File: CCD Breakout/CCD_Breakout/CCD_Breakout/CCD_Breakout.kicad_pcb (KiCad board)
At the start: 2 copper layers, 80.5 x 25.4 mm, 33 parts, among them U1 CCD, U3 ADC-MCP33151, U5 74HC541PW_118, U8 OPA4322AIPWR

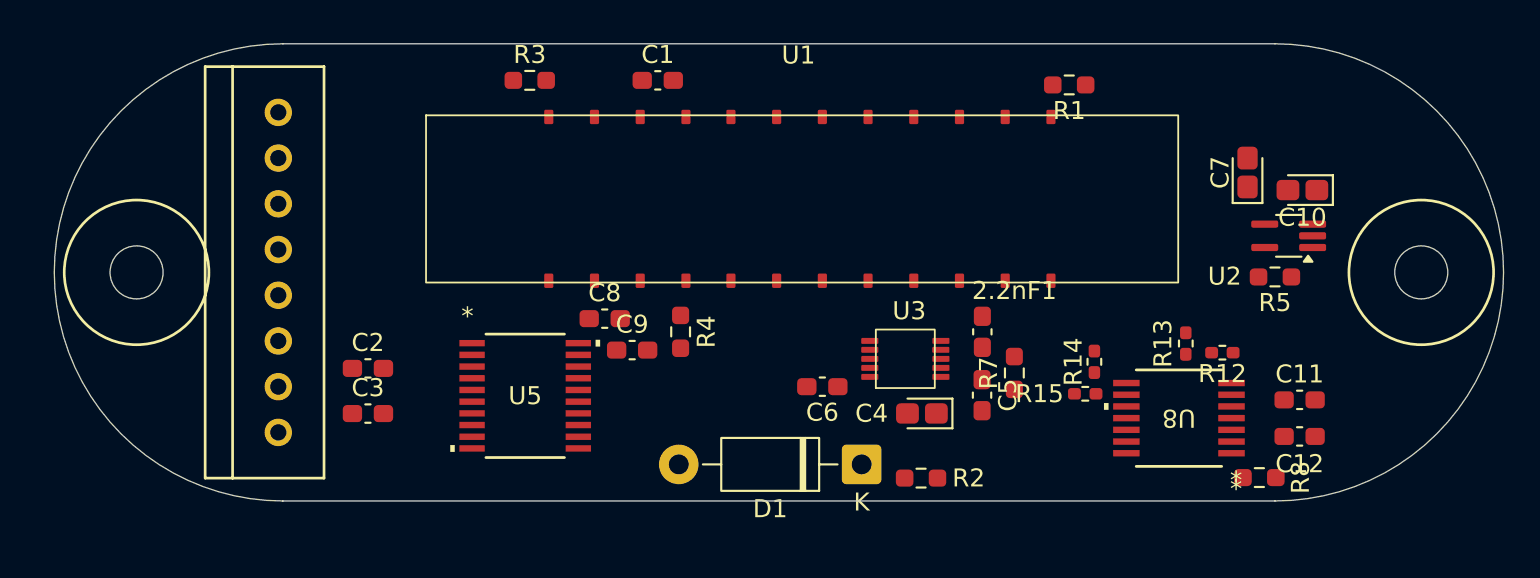
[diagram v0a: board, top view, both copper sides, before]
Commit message: CCD Layout Traces
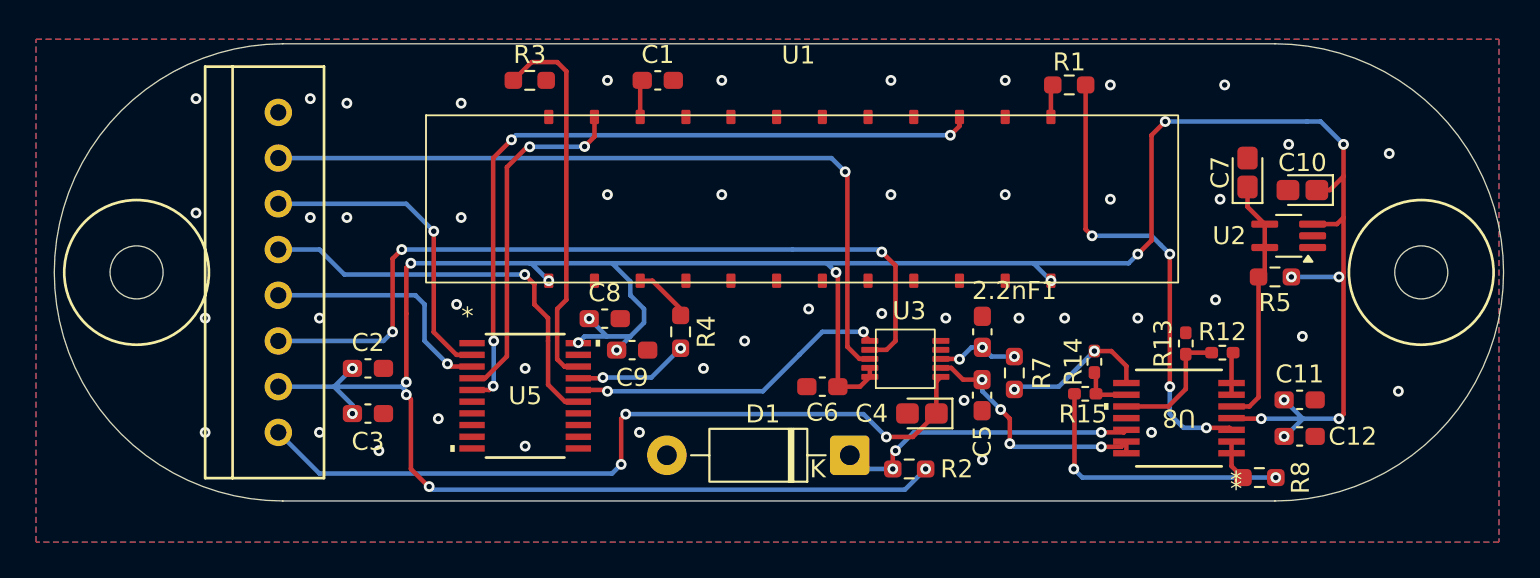
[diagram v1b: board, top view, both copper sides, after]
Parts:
- moved D1 0.83 mm to (149.4, 96.8)
- moved R2 0.83 mm to (152.7, 97.5)
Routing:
- net +5V: track 0.00 -> 164.6 mm, vias 0 -> 22
- net /ADC/OUT: track 0.00 -> 45.0 mm, vias 0 -> 3
- net +3V3: track 0.00 -> 43.6 mm, vias 0 -> 3
- net /ADC/CLK2: track 0.00 -> 43.1 mm, vias 0 -> 1
- net /CCD/EOSb: track 0.00 -> 41.1 mm, vias 0 -> 4
- net /CCD/opINA+: track 0.00 -> 25.9 mm, vias 0 -> 4
- net /CCD/EOS: track 0.00 -> 23.0 mm, vias 0 -> 1
- net /CCD/STb: track 0.00 -> 21.1 mm
- net /CCD/Trigb: track 0.00 -> 19.6 mm, vias 0 -> 2
- net /ADC/TRIG: track 0.00 -> 17.9 mm, vias 0 -> 2
- net /CCD/ST: track 0.00 -> 17.5 mm, vias 0 -> 1
- net /ADC/opIND+: track 0.00 -> 17.1 mm, vias 0 -> 3
- net /CCD/Videob: track 0.00 -> 15.6 mm, vias 0 -> 2
- net /ADC/opIND-: track 0.00 -> 14.1 mm, vias 0 -> 4
- net /CCD/opINB+: track 0.00 -> 13.9 mm
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- added copper zone on B.Cu, net GND
- added copper zone on F.Cu, net GND
